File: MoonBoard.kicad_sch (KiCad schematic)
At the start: 19 parts, among them SW1 SW_SPST, U1 AMS1117-3.3, U2 STM32F446RETx, Y1 25MHz

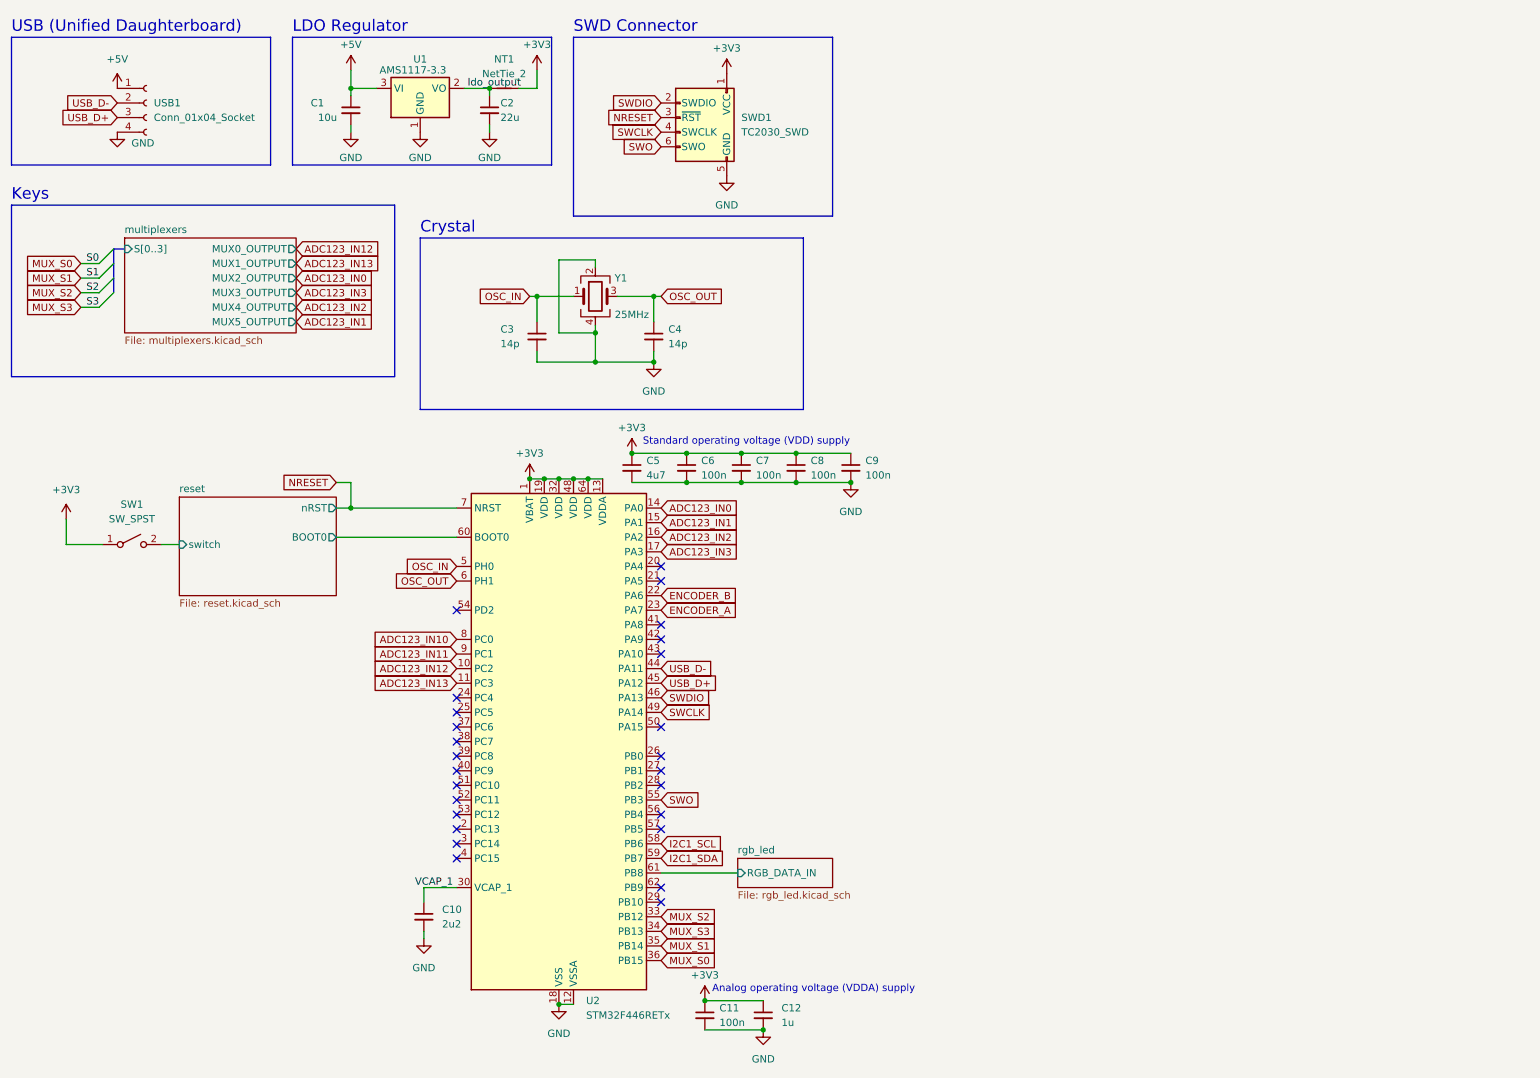
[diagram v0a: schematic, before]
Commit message: usb hub awfulness
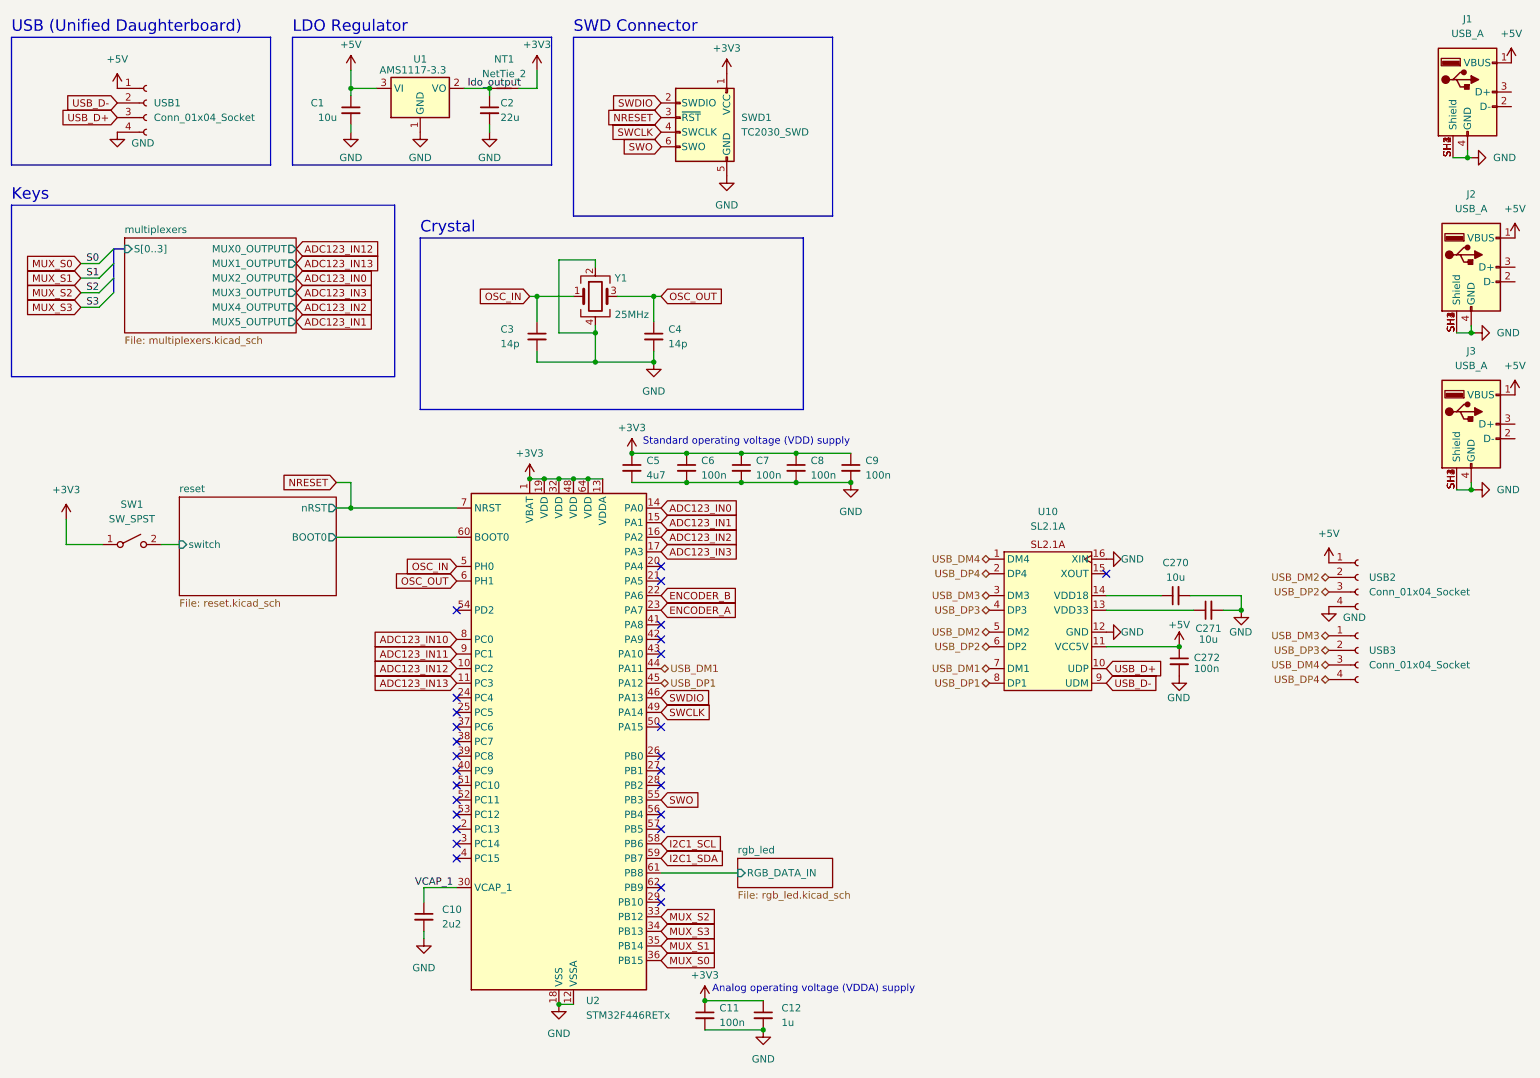
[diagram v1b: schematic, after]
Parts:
- added C270, C271: 10u, symbol Device:C_Small
- added C272: 100n, Capacitor_SMD:C_0402_1005Metric, symbol Device:C_Small
- added J1, J2, J3: USB_A, MoonBoard:USB-A-SMD_AF-APPLE-10.6, symbol Connector:USB_A
- added U10: SL2.1A, MoonBoard:SSOP-16_L4.6-W2.6-P0.53-LS4.0-BL, symbol MoonBoard:SL2.1A
- added USB2, USB3: Conn_01x04_Socket, Connector_Molex:Molex_Pico-EZmate_78171-0004_1x04-1MP_P1.20mm_Vertical, symbol Connector:Conn_01x04_Socket
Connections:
- net +5V: now also C272.1, J1.1 (VBUS), J2.1 (VBUS), J3.1 (VBUS), U10.11 (VCC5V), USB2.1 (Pin_1)
- net GND: now also C270.2, C271.2, C272.2, J1.4 (GND), J1.SH1 (Shield), J1.SH2 (Shield), J1.SH3 (Shield), J1.SH4 (Shield), J2.4 (GND), J2.SH1 (Shield), J2.SH2 (Shield), J2.SH3 (Shield), J2.SH4 (Shield), J3.4 (GND), J3.SH1 (Shield), J3.SH2 (Shield), J3.SH3 (Shield), J3.SH4 (Shield), U10.12 (GND), U10.16 (XIN), USB2.4 (Pin_4)
- net USB_D+: now also U10.10 (UDP); no longer U2.45 (PA12)
- net USB_D-: now also U10.9 (UDM); no longer U2.44 (PA11)
- new net: C271.1, U10.13 (VDD33)
- new net: C270.1, U10.14 (VDD18)
- new net USB_DM1: U10.7 (DM1), U2.44 (PA11)
- new net USB_DM2: U10.5 (DM2), USB2.2 (Pin_2)
- new net USB_DM3: U10.3 (DM3), USB3.1 (Pin_1)
- new net USB_DM4: U10.1 (DM4), USB3.3 (Pin_3)
- new net USB_DP1: U10.8 (DP1), U2.45 (PA12)
- new net USB_DP2: U10.6 (DP2), USB2.3 (Pin_3)
- new net USB_DP3: U10.4 (DP3), USB3.2 (Pin_2)
- new net USB_DP4: U10.2 (DP4), USB3.4 (Pin_4)
- no-connect marks 26 -> 27
